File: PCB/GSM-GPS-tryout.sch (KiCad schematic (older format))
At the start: 6 parts, among them J7 Jack-DC

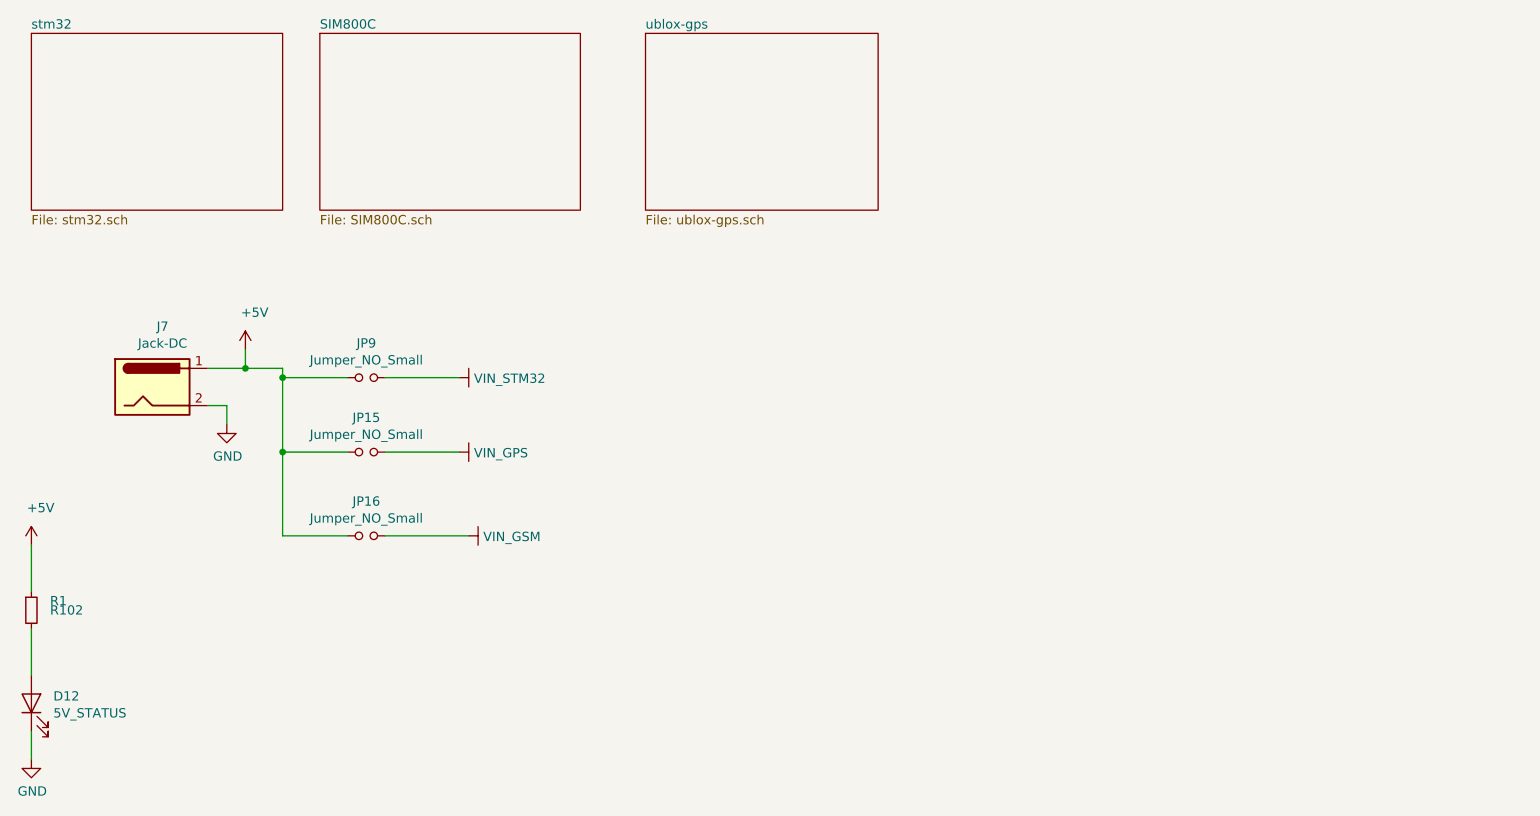
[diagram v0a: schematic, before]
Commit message: updte
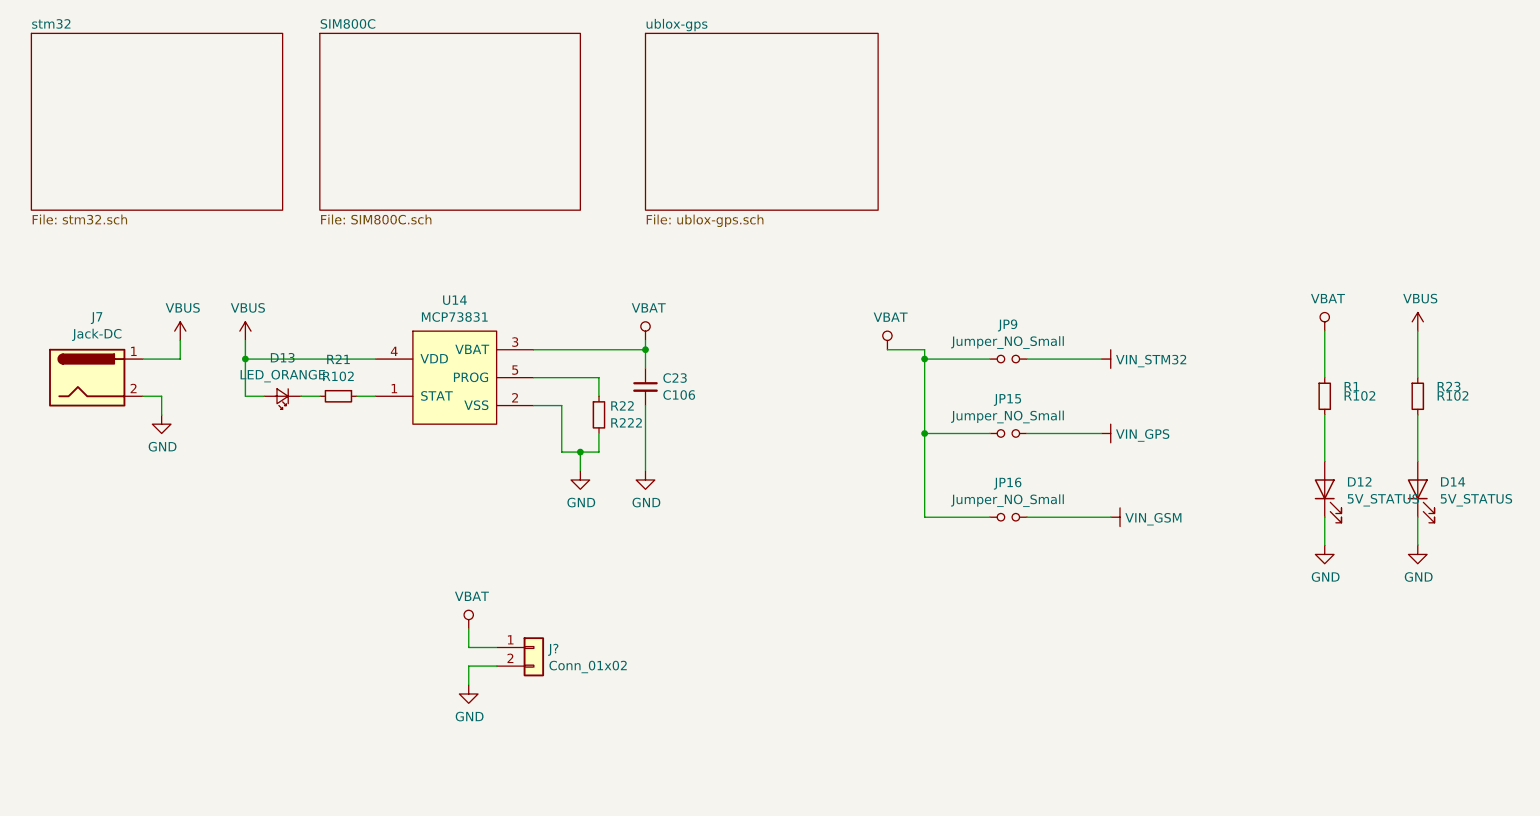
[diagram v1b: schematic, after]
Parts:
- added C23: C106, Capacitor_SMD:C_0805_2012Metric_Pad1.15x1.40mm_HandSolder, symbol taobao-c:C106
- added D13: LED_ORANGE, LED_SMD:LED_0805_2012Metric_Castellated, symbol taobao-components:LED_GREEN
- added D14: 5V_STATUS, LED_SMD:LED_0805_2012Metric_Pad1.15x1.40mm_HandSolder, symbol Device:LED
- added J?: Conn_01x02, symbol Connector_Generic:Conn_01x02
- added R21, R23: R102, Resistor_SMD:R_0805_2012Metric_Pad1.15x1.40mm_HandSolder, symbol taobao-r:R102
- added R22: R222, Resistor_SMD:R_0805_2012Metric_Pad1.15x1.40mm_HandSolder, symbol taobao-r:R222
- added U14: MCP73831, Package_TO_SOT_SMD:SOT-23-5_HandSoldering, symbol taobao-components:MCP73831
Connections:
- net GND: now also C23.2, D14.1 (K), J?.2 (Pin_2), R22.2, U14.2 (VSS)
- net +5V renamed VBAT
- net VBAT: now also C23.1, J?.1 (Pin_1), U14.3 (VBAT); no longer J7.1
- new net: D13.1 (K), R21.2
- new net: R21.1, U14.1 (STAT)
- new net: R22.1, U14.5 (PROG)
- new net: D14.2 (A), R23.2
- new net VBUS: D13.2 (A), J7.1, R23.1, U14.4 (VDD)
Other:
- moved on the sheet: D12, J7, JP15, JP16, JP9, R1
